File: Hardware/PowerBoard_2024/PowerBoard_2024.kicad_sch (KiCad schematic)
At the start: 220 parts, among them J1 RJ45_LED_Shielded, Q1 BSS138, Q10 BSS138, Q11 BSS138, Q12 IRF7606PBF, Q13 IRF7606PBF, Q14 SPD30P06PGBTMA1, Q15 BSS138, Q16 SPD30P06PGBTMA1, Q17 BSS138, Q18 BSS138, Q19 BSS138, Q2 IRF7606PBF, Q20 IRF7606PBF, Q21 IRF7606PBF, Q22 SPD30P06PGBTMA1, Q23 BSS138, Q24 SPD30P06PGBTMA1, Q25 BSS138, Q26 SPD30P06PGBTMA1, Q27 BSS138, Q28 SPD30P06PGBTMA1, Q29 BSS138, Q3 BSS138, Q30 SPD30P06PGBTMA1, Q4 IRF7606PBF, Q5 BSS138, Q6 SPD30P06PGBTMA1, Q7 BSS138, Q8 SPD30P06PGBTMA1, Q9 BSS138, U1 3V3, U10 ACS725xLCTR-20AB, U11 ACS725xLCTR-20AB, U12 ACS725xLCTR-20AB, U13 ACS725xLCTR-20AB, U14 ACS725xLCTR-20AB, U15 Teensy4.1_DEV-16771, U16 ACS725xLCTR-20AB, U17 ACS725xLCTR-20AB, U18 ACS725xLCTR-20AB, U19 ACS725xLCTR-20AB, U2 ACS725xLCTR-20AB, U20 PKE3316ZPI, U21 ACS725xLCTR-20AB, U22 PKE3316ZPI, U23 ACS725xLCTR-20AB, U3 ACS725xLCTR-20AB, U4 ACS725xLCTR-20AB, U5 ACS725xLCTR-20AB, U6 ACS725xLCTR-20AB, U7 ACS725xLCTR-20AB, U8 ACS725xLCTR-20AB, U9 ACS725xLCTR-20AB

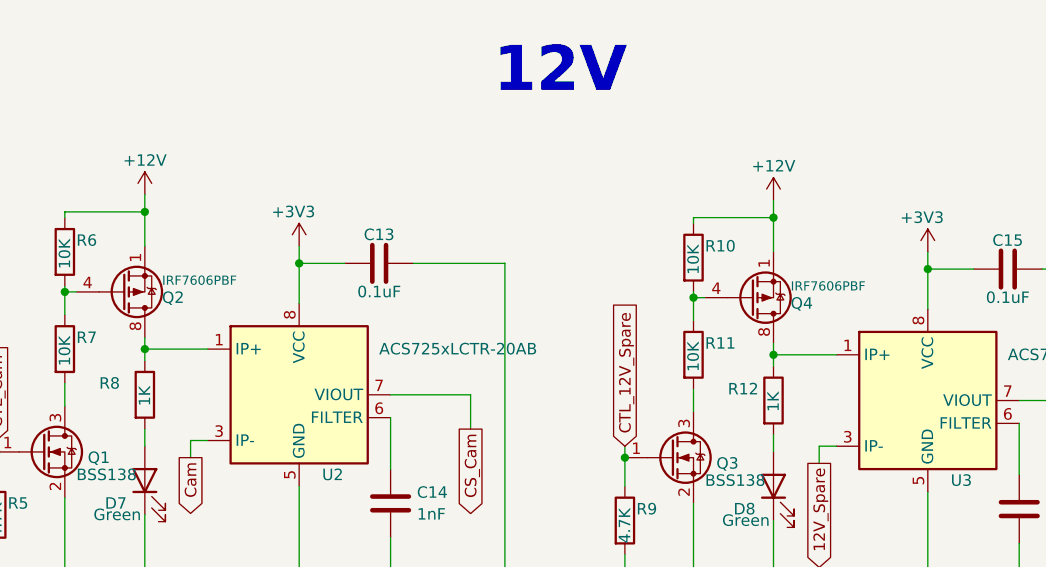
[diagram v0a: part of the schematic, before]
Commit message: Rev 1 Layout Orgainization
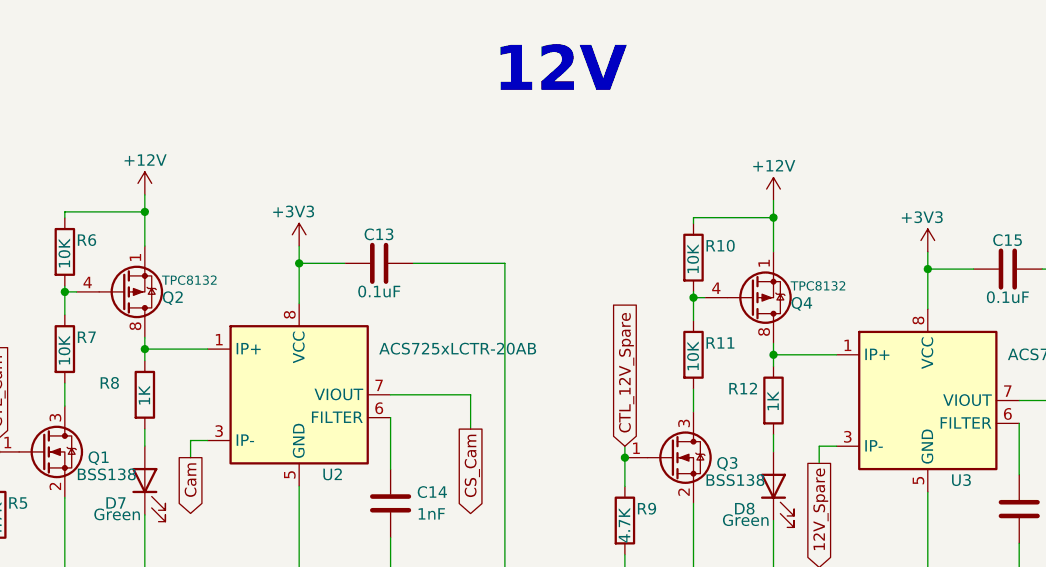
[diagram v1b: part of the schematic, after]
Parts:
- Q2, Q4: value IRF7606PBF -> TPC8132; footprint Package_SO:MSOP-8_3x3mm_P0.65mm -> Package_SO:SOP-8_3.9x4.9mm_P1.27mm
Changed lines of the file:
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@@
       (effects (font (size 1.27 1.27)) (justify left))
     )
-    (property "Value" "IRF7606PBF" (at 234.95 176.53 0)
+    (property "Value" "TPC8132" (at 234.95 176.53 0)
       (effects (font (size 1.016 1.016)) (justify left))
     )
-    (property "Footprint" "Package_SO:MSOP-8_3x3mm_P0.65mm" (at 235.585 175.895 0)
+    (property "Footprint" "Package_SO:SOP-8_3.9x4.9mm_P1.27mm" (at 235.585 175.895 0)
       (effects (font (size 1.27 1.27) italic) (justify left) hide)
     )
@@
       (effects (font (size 1.27 1.27)) (justify left))
     )
-    (property "Value" "IRF7606PBF" (at 165.1 175.895 0)
+    (property "Value" "TPC8132" (at 165.1 175.895 0)
       (effects (font (size 1.016 1.016)) (justify left))
     )
-    (property "Footprint" "Package_SO:MSOP-8_3x3mm_P0.65mm" (at 165.735 175.26 0)
+    (property "Footprint" "Package_SO:SOP-8_3.9x4.9mm_P1.27mm" (at 165.735 175.26 0)
       (effects (font (size 1.27 1.27) italic) (justify left) hide)
     )

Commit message: Layout Traces
Finished Trace Work
Added Signature
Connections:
- net Aux: now also Conn9.4 (PV+), U5.3 (IP-), U5.4 (IP-); no longer Conn8.4 (PV+), U9.3 (IP-), U9.4 (IP-)
- net CS_Aux: now also U15.20 (A6), U5.7 (VIOUT); no longer U15.19 (A5), U9.7 (VIOUT)
- net CS_Cam: now also U15.18 (A4); no longer U15.17 (A3)
- net CS_Core: now also U15.39 (A15); no longer U15.22 (A8)
- net CS_DiffGPS: now also U15.40 (A16); no longer U15.21 (A7)
- net CS_HC_Spare: now also U15.19 (A5), U9.7 (VIOUT); no longer U15.18 (A4), U5.7 (VIOUT)
- net CS_LC_Spare: now also U15.38 (A14); no longer U15.23 (A9)
- net CS_M1: now also U15.21 (A7); no longer U15.38 (A14)
- net CS_M2: now also U15.22 (A8); no longer U15.39 (A15)
- net CS_M3: now also U15.23 (A9); no longer U15.40 (A16)
- net CS_M4: now also U15.24 (A10); no longer U15.41 (A17)
- net CS_M5: now also U15.25 (A11); no longer U15.14 (A0)
- net CS_M6: now also U15.26 (A12); no longer U15.15 (A1)
- net CS_MS: now also U15.27 (A13); no longer U15.16 (A2)
- net CS_Net Switch_1: now also U15.17 (A3); no longer U15.24 (A10)
- net CS_Net Switch_2: now also U15.16 (A2); no longer U15.25 (A11)
- net CS_Net Switch_3: now also U15.15 (A1); no longer U15.26 (A12)
- net CS_POE: now also U15.14 (A0); no longer U15.27 (A13)
- net CS_RouterPi: now also U15.41 (A17); no longer U15.20 (A6)
- net CTL_Aux: now also Q7.1 (G), R17.1, U15.29 (TX7); no longer Q15.1 (G), R33.1, U15.5 (IN2)
- net CTL_Cam: now also U15.10 (CS1); no longer U15.7 (RX2)
- net CTL_Core: now also U15.36 (CS2); no longer U15.10 (CS1)
- net CTL_DiffGPS: now also U15.35 (TX8); no longer U15.11 (MOSI)
- net CTL_HC_Spare: now also Q15.1 (G), R33.1, U15.30 (CRX3); no longer Q7.1 (G), R17.1, U15.6 (OUT1D)
- net CTL_LC_Spare: now also U15.37 (CS3); no longer U15.9 (OUT1C)
- net CTL_M1: now also U15.28 (RX7); no longer U15.34 (RX8)
- net CTL_M2: now also U15.12 (MISO); no longer U15.35 (TX8)
- net CTL_M3: now also U15.11 (MOSI); no longer U15.36 (CS2)
- net CTL_M4: now also U15.5 (IN2); no longer U15.37 (CS3)
- net CTL_M5: now also U15.6 (OUT1D); no longer U15.30 (CRX3)
- net CTL_M6: now also U15.7 (RX2); no longer U15.29 (TX7)
- net CTL_MS: now also U15.9 (OUT1C); no longer U15.28 (RX7)
- net CTL_RouterPi: now also U15.34 (RX8); no longer U15.12 (MISO)
- net HC_Spare: now also Conn8.4 (PV+), U9.3 (IP-), U9.4 (IP-); no longer Conn9.4 (PV+), U5.3 (IP-), U5.4 (IP-)
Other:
- moved on the sheet: Q15

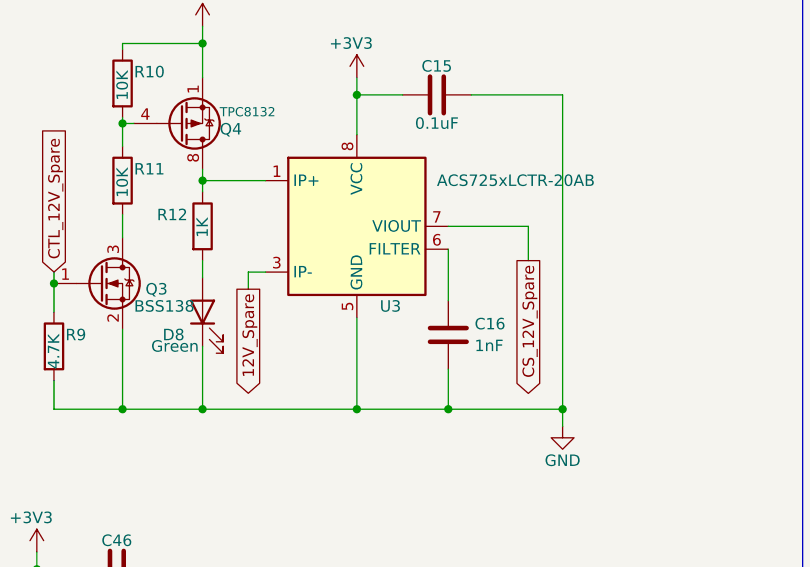
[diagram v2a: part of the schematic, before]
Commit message: Finished Third Review Layout
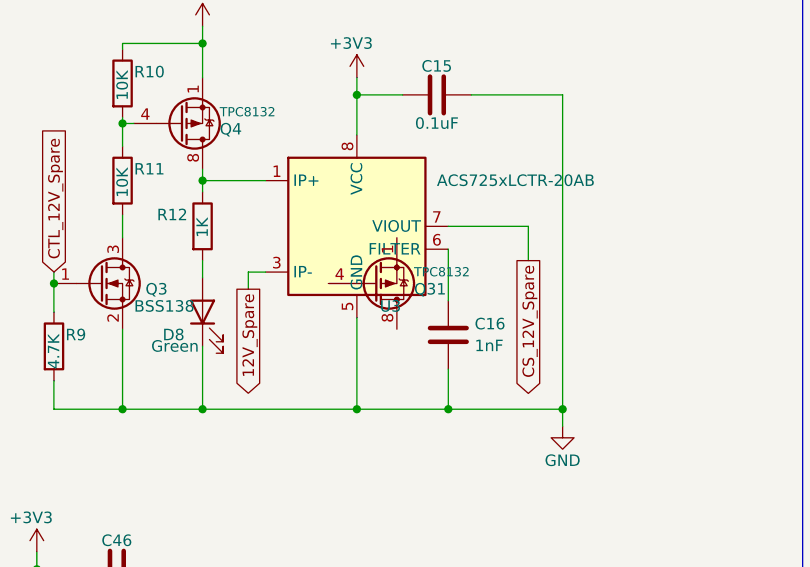
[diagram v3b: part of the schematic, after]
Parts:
- added Q31: TPC8132, Package_SO:MSOP-8_3x3mm_P0.65mm, symbol Transistor_FET:IRF7606PBF
- Q2, Q4: footprint Package_SO:SOP-8_3.9x4.9mm_P1.27mm -> Package_SO:MSOP-8_3x3mm_P0.65mm
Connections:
- new net: Q31.1 (S), Q31.2 (S), Q31.3 (S)
- new net: Q31.5 (D), Q31.6 (D), Q31.7 (D), Q31.8 (D)
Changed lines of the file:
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@@
     )
   )
+  (symbol (lib_id "Transistor_FET:IRF7606PBF") (at 252.095 195.58 0) (mirror x) (unit 1)
+    (in_bom yes) (on_board yes) (dnp no)
+    (property "Reference" "Q31" (at 256.54 196.215 0)
+      (effects (font (size 1.27 1.27)) (justify left))
+    )
+    (property "Value" "TPC8132" (at 256.54 194.31 0)
+      (effects (font (size 1.016 1.016)) (justify left))
+    )
+    (property "Footprint" "Package_SO:MSOP-8_3x3mm_P0.65mm" (at 257.175 193.675 0)
+      (effects (font (size 1.27 1.27) italic) (justify left) hide)
+    )
+    (property "Datasheet" "http://www.irf.com/product-info/datasheets/data/irf7606pbf.pdf" (at 252.095 195.58 90)
+      (effects (font (size 1.27 1.27)) (justify left) hide)
+    )
+    (pin "1")
+    (pin "2")
+    (pin "3")
+    (pin "4")
+    (pin "5")
+    (pin "6")
+    (pin "7")
+    (pin "8")
+    (instances
+      (project "PowerBoard_2024"
+        (path "/8ad22d76-a558-4ba1-aeeb-dc7eabdc9e9b"
+          (reference "Q31") (unit 1)
+        )
+      )
+    )
+  )
   (symbol (lib_id "Device:R") (at 470.535 104.775 0) (unit 1)
     (in_bom yes) (on_board yes) (dnp no)
@@
       (effects (font (size 1.016 1.016)) (justify left))
     )
-    (property "Footprint" "Package_SO:SOP-8_3.9x4.9mm_P1.27mm" (at 235.585 175.895 0)
+    (property "Footprint" "Package_SO:MSOP-8_3x3mm_P0.65mm" (at 235.585 175.895 0)
       (effects (font (size 1.27 1.27) italic) (justify left) hide)
     )
@@
       (effects (font (size 1.016 1.016)) (justify left))
     )
-    (property "Footprint" "Package_SO:SOP-8_3.9x4.9mm_P1.27mm" (at 165.735 175.26 0)
+    (property "Footprint" "Package_SO:MSOP-8_3x3mm_P0.65mm" (at 165.735 175.26 0)
       (effects (font (size 1.27 1.27) italic) (justify left) hide)
     )
